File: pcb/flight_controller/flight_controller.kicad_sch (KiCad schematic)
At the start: 5 parts, among them U1 ICM-42688-P, U2 STM32F405RGT6

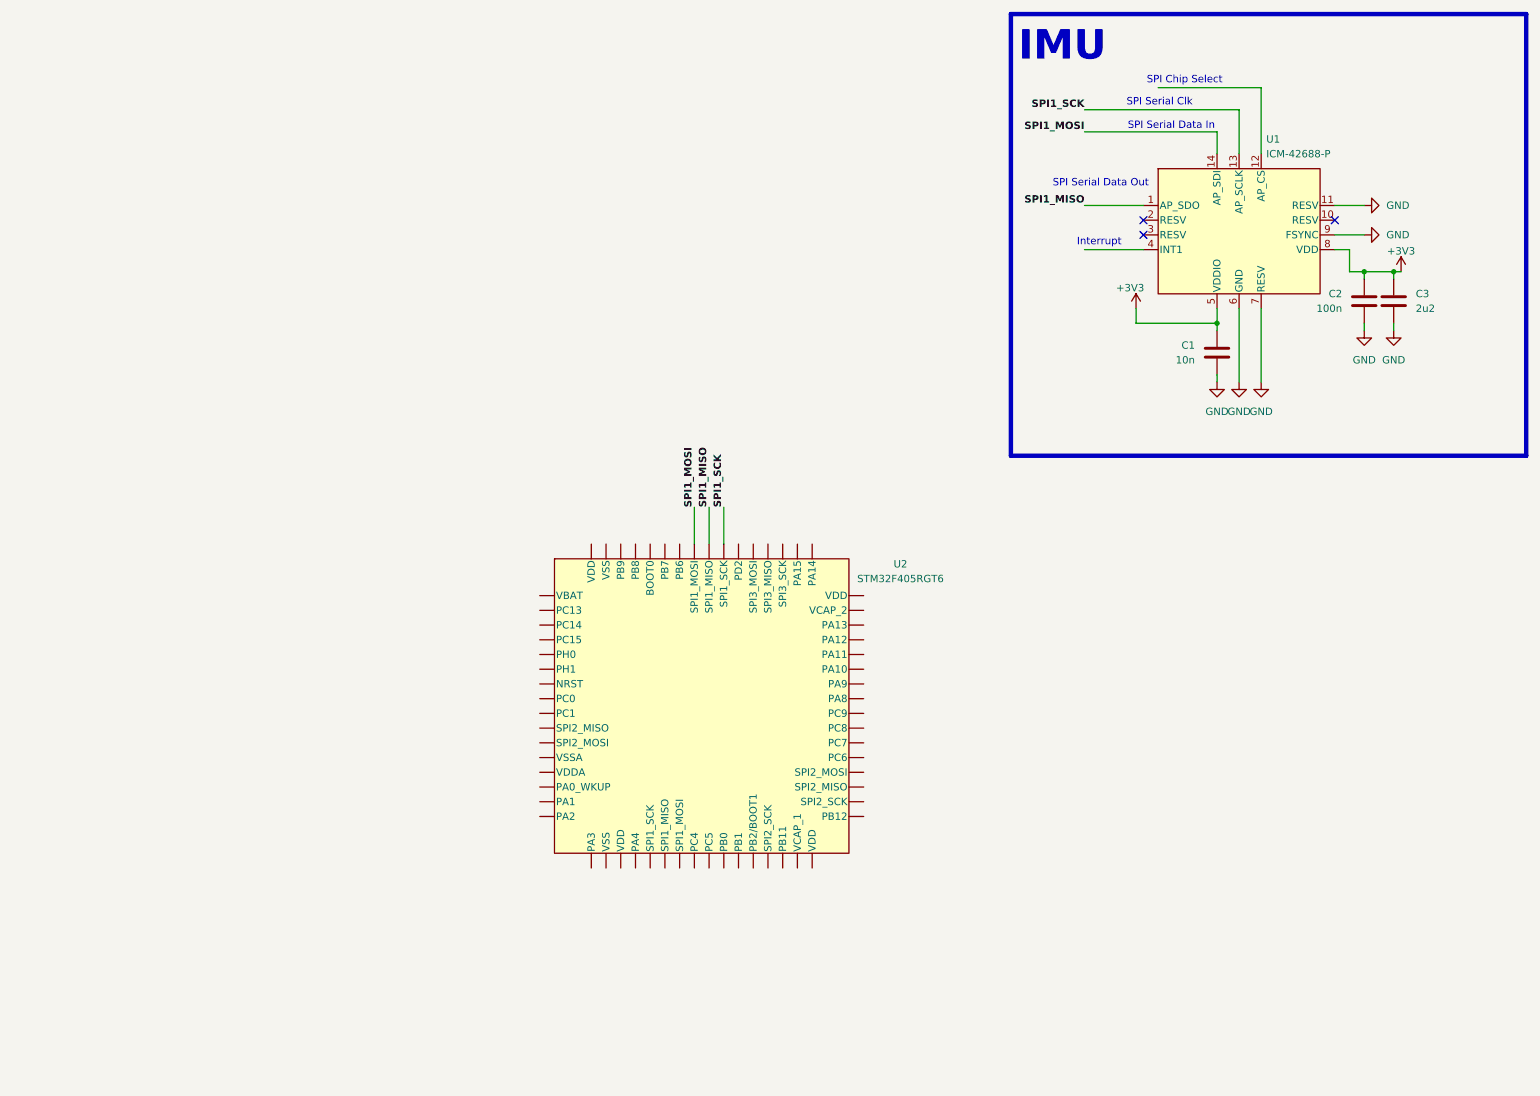
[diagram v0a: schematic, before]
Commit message: added some datasheets and did some work on the mcu
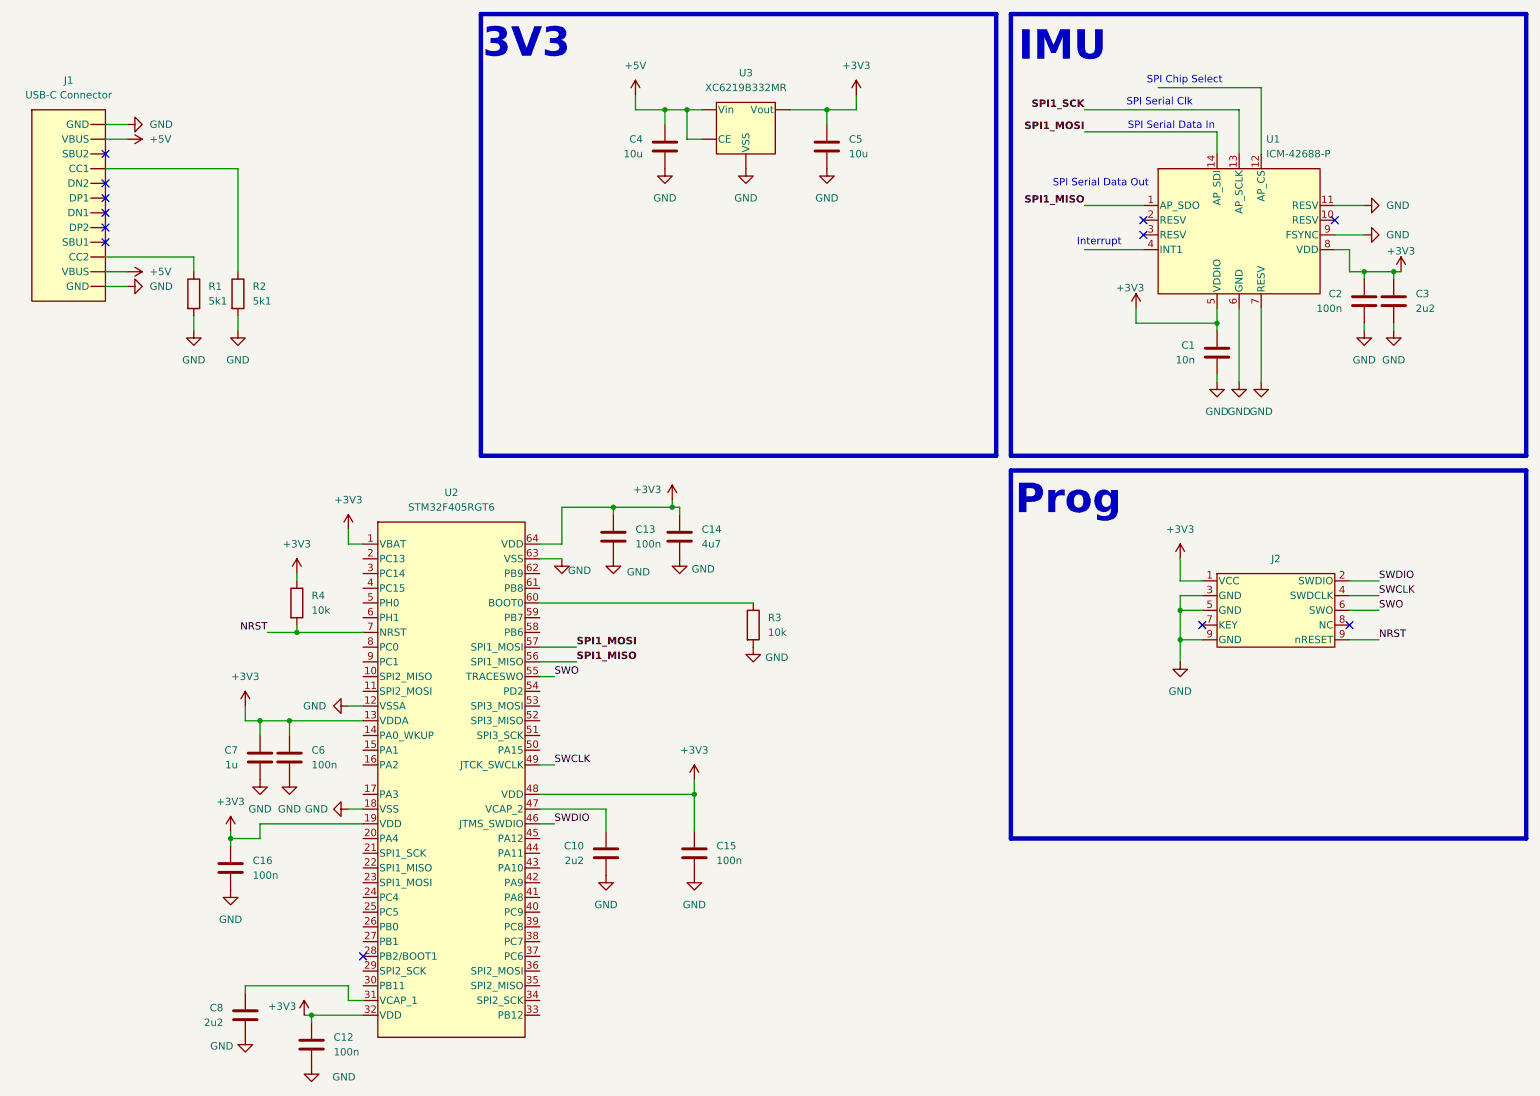
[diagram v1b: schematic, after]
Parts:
- added C10, C8: 2u2, symbol Device:C
- added C12, C13, C15, C16, C6: 100n, symbol Device:C
- added C14: 4u7, symbol Device:C
- added C4, C5: 10u, symbol Device:C
- added C7: 1u, symbol Device:C
- added J1: USB-C Connector, symbol symbols_local:USB-C_Vertical_12pin
- added J2: (no value), symbol symbols_local:SWD_Header
- added R1, R2: 5k1, symbol Device:R
- added R3, R4: 10k, symbol Device:R
- added U3: XC6219B332MR, symbol symbols_local:XC6219B332MR
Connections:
- net +3V3: now also U2.1 (VBAT), U2.13 (VDDA), U2.19 (VDD), U2.32 (VDD), U2.48 (VDD), U2.64 (VDD), C12.2, C13.2, C14.2, C15.2, C16.2, C5.2, C6.2, C7.2, J2.1 (VCC), R4.1, U3.5 (Vout)
- net GND: now also U2.12 (VSSA), U2.18 (VSS), U2.63 (VSS), C10.1, C12.1, C13.1, C14.1, C15.1, C16.1, C4.1, C5.1, C6.1, C7.1, C8.1, J1.1 (GND), J1.12 (GND), J2.3 (GND), J2.5 (GND), J2.9 (nRESET), R1.2, R2.2, R3.2, U3.2 (VSS)
- net SPI1_SCK: no longer U2.55 (PB3)
- net at U2.31 (VCAP_1): now also C8.2
- net SWDIO: now reaches U2.46 (PA13)
- net SWDIO: now also J2.2 (SWDIO)
- net at U2.47 (VCAP_2): now also C10.2
- net SWCLK: now reaches U2.49 (PA14)
- net SWCLK: now also J2.4 (SWDCLK)
- net at U2.60 (BOOT0): now also R3.1
- net NRST: now reaches U2.7 (NRST)
- net NRST: now also J2.9 (nRESET), R4.2
- new net: J1.4 (CC1), R2.1
- new net: J1.10 (CC2), R1.1
- new net +5V: C4.2, J1.11 (VBUS), J1.2 (VBUS), U3.1 (Vin), U3.3 (CE)
- new net SWO: J2.6 (SWO), U2.55 (PB3)
- no-connect marks 3 -> 12
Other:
- note added: "3V3"
- note added: "Prog"
